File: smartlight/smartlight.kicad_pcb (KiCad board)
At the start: 2 copper layers, 43 x 36 mm, 20 parts, among them J1 Conn_01x06, J2 Conn_01x05, U1 ESP-12F

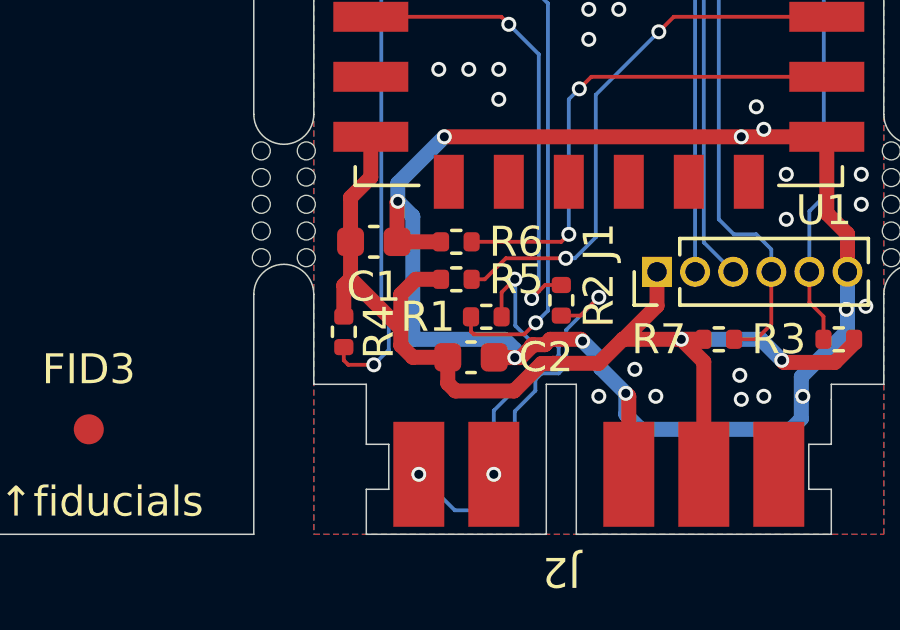
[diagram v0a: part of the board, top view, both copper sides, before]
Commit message: update
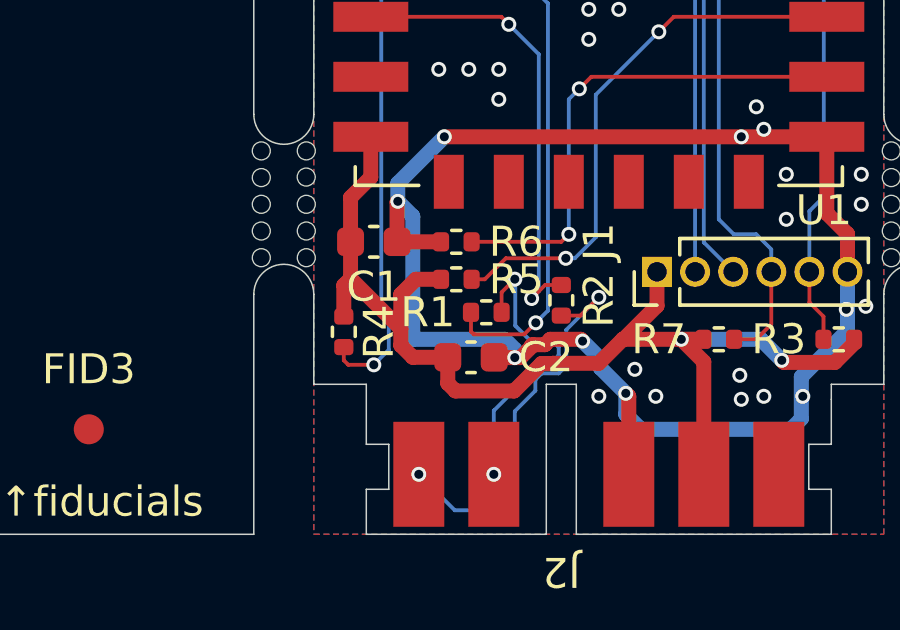
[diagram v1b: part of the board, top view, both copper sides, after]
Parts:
- moved R1 0.15 mm to (86.2, 66.1)
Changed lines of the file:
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@@
 		(tags "capacitor")
 		(property "Reference" "C2"
-			(at 2.5 0 360)
+			(at 2.5 0 0)
 			(layer "F.SilkS")
 			(effects
@@
 		)
 		(property "Value" "1u"
-			(at 0 1.43 360)
+			(at 0 1.43 0)
 			(layer "F.Fab")
 			(effects
@@
 		)
 		(fp_text user "${REFERENCE}"
-			(at 0 0 360)
+			(at 0 0 0)
 			(layer "F.Fab")
 			(effects
@@
 	(footprint "Resistor_SMD:R_0402_1005Metric"
 		(layer "F.Cu")
-		(at 86.25 66.25)
+		(at 86.25 66.1)
 		(descr "Resistor SMD 0402 (1005 Metric), square (rectangular) end terminal, IPC_7351 nominal, (Body size source: IPC-SM-782 page 72, https://www.pcb-3d.com/wordpress/wp-content/uploads/ipc-sm-782a_amendment_1_and_2.pdf), generated with kicad-footprint-generator")
 		(tags "resistor")
 		(property "Reference" "R1"
-			(at -1.95 0 360)
+			(at -1.95 0 0)
 			(layer "F.SilkS")
 			(effects
@@
 		)
 		(property "Value" "100"
-			(at 0 1.17 360)
+			(at 0 1.17 0)
 			(layer "F.Fab")
 			(effects
@@
 		)
 		(fp_text user "${REFERENCE}"
-			(at 0 0 360)
-			(layer "F.Fab")
-			(effects
+			(at 0 0 0)
+			(layer "F.Fab")
+			(effects
